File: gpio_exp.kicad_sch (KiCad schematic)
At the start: 22 parts, among them U11 MCP23S17_SO

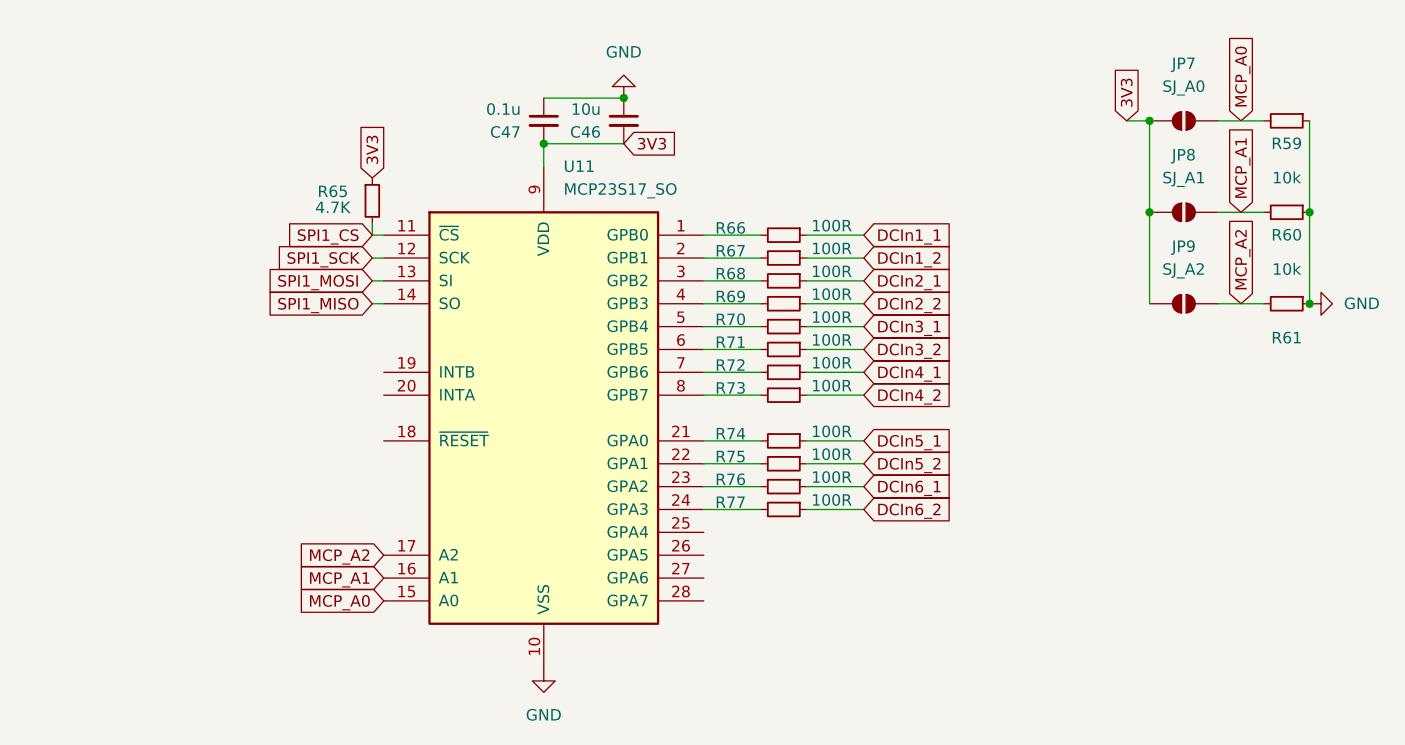
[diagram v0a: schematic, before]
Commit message: Visual Improvements
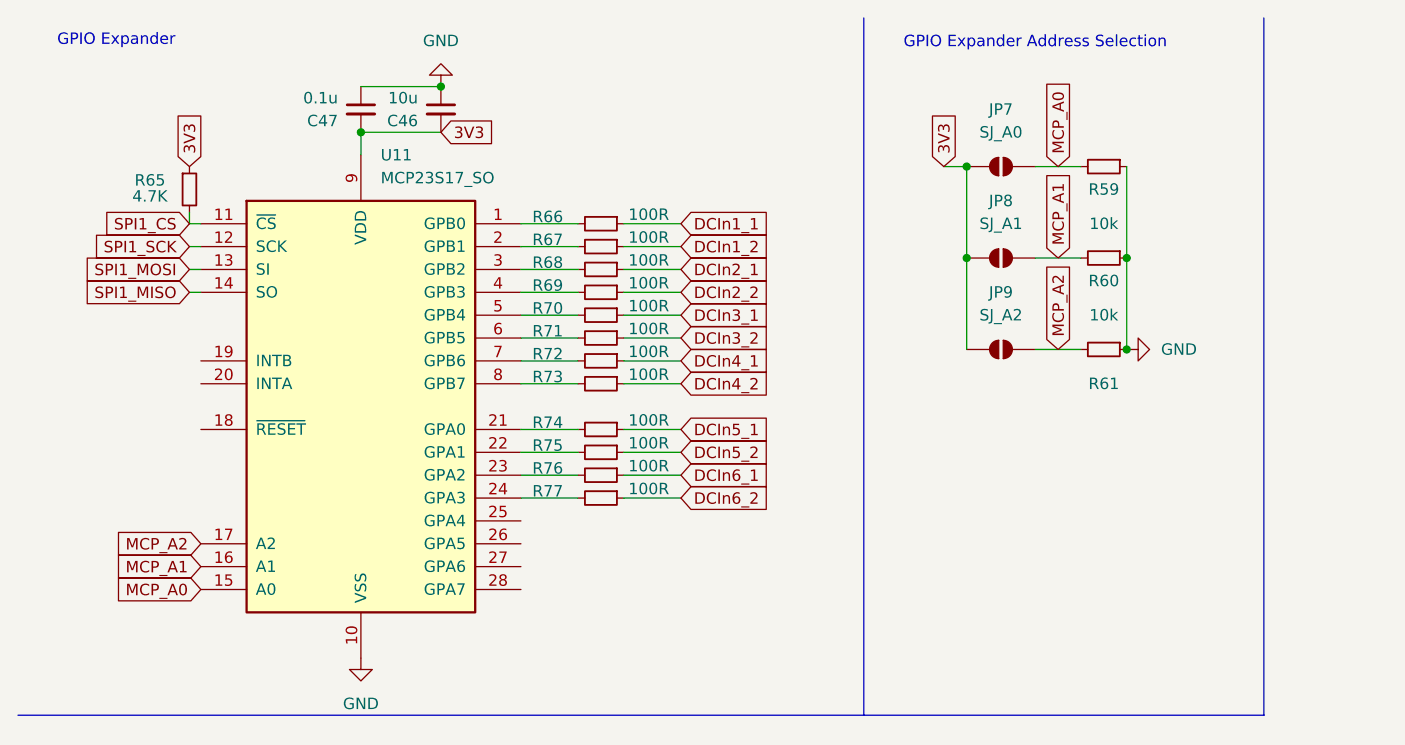
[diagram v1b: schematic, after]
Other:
- note added: "GPIO Expander"
- note added: "GPIO Expander Address Selection"
- moved on the sheet: C46, C47, JP7, JP8, JP9, R59, R60, R61, R65, R66, R67, R68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
